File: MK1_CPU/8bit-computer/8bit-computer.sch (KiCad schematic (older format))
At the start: 16 parts, among them J1 USB_B-8bit-computer-rescue, J2 Barrel_Jack_Switch, U1 74HCT32, U2 74HCT32

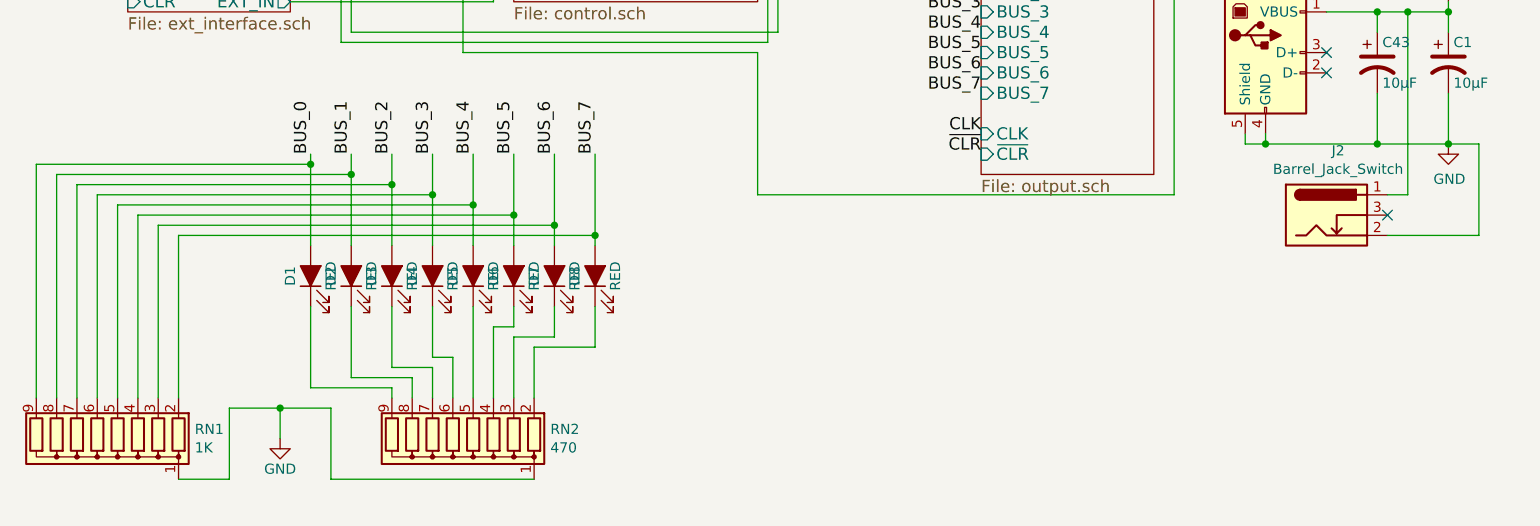
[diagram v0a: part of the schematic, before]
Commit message: 2.0b hardware revision
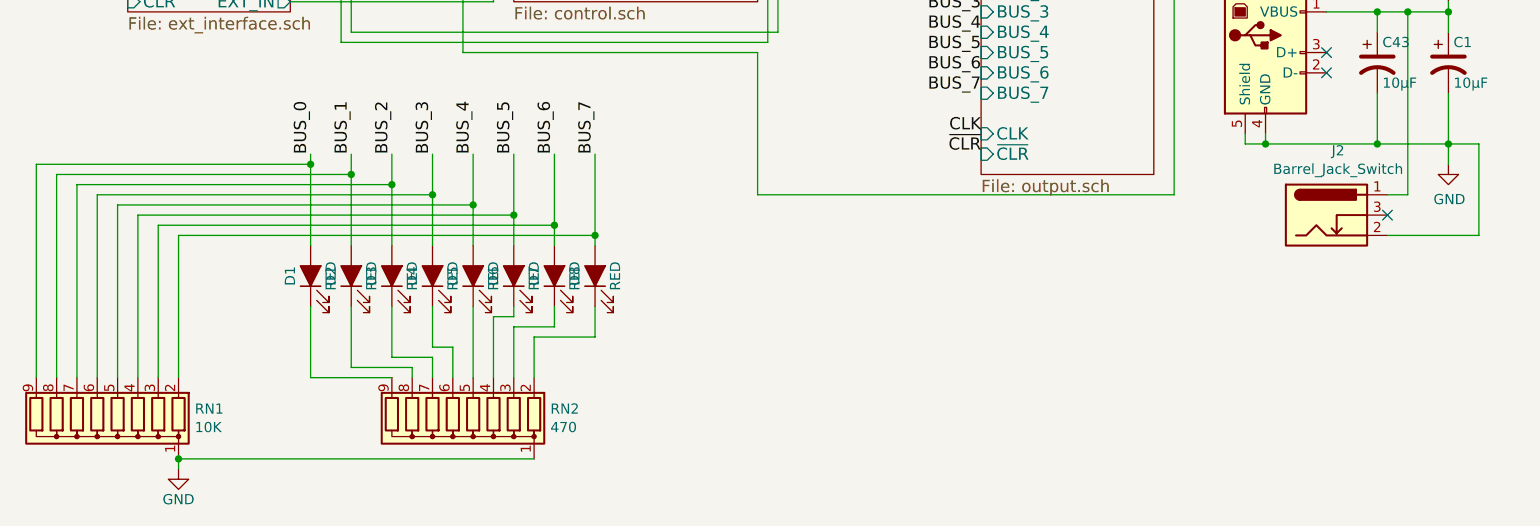
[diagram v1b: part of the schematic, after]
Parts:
- RN1: value 1K -> 10K
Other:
- moved on the sheet: RN1, RN2
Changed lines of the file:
@@
 L power:GND #PWR01
 U 1 1 5B60DD27
-P 1800 10850
-F 0 "#PWR01" H 1800 10600 50  0001 C CNN
-F 1 "GND" H 1800 10700 50  0000 C CNN
-F 2 "" H 1800 10850 50  0001 C CNN
-F 3 "" H 1800 10850 50  0001 C CNN
-	1    1800 10850
+P 1300 11000
+F 0 "#PWR01" H 1300 10750 50  0001 C CNN
+F 1 "GND" H 1300 10850 50  0000 C CNN
+F 2 "" H 1300 11000 50  0001 C CNN
+F 3 "" H 1300 11000 50  0001 C CNN
+	1    1300 11000
 	1    0    0    -1
 $EndComp
-Wire Wire Line
-	1800 10850 1800 10700
 Wire Wire Line
 	2350 9600 2350 9900
@@
 L power:GND #PWR03
 U 1 1 5E907257
-P 7550 9400
-F 0 "#PWR03" H 7550 9150 50  0001 C CNN
-F 1 "GND" H 7555 9227 50  0000 C CNN
-F 2 "" H 7550 9400 50  0001 C CNN
-F 3 "" H 7550 9400 50  0001 C CNN
-	1    7550 9400
+P 7550 9500
+F 0 "#PWR03" H 7550 9250 50  0001 C CNN
+F 1 "GND" H 7555 9327 50  0000 C CNN
+F 2 "" H 7550 9500 50  0001 C CNN
+F 3 "" H 7550 9500 50  0001 C CNN
+	1    7550 9500
 	1    0    0    -1
 $EndComp
@@
 Wire Wire Line
 	650  5200 950  5200
-$Comp
-L Device:R_Network08 RN2
-U 1 1 76216E60
-P 2650 10850
-F 0 "RN2" H 2170 10804 50  0000 R CNN
-F 1 "470" H 2170 10895 50  0000 R CNN
-F 2 "Resistor_THT:R_Array_SIP9" V 3125 10850 50  0001 C CNN
-F 3 "http://www.vishay.com/docs/31509/csc.pdf" H 2650 10850 50  0001 C CNN
-	1    2650 10850
-	-1   0    0    1
-$EndComp
-Wire Wire Line
-	3050 11050 2050 11050
-Wire Wire Line
-	2050 11050 2050 10700
-Wire Wire Line
-	2050 10700 1800 10700
-Wire Wire Line
-	1950 10600 2350 10600
-Wire Wire Line
-	2350 10600 2350 10650
-Wire Wire Line
-	1950 10200 1950 10600
-Wire Wire Line
-	2150 10550 2450 10550
-Wire Wire Line
-	2450 10550 2450 10650
-Wire Wire Line
-	2150 10200 2150 10550
-Wire Wire Line
-	2350 10500 2550 10500
-Wire Wire Line
-	2550 10500 2550 10650
-Wire Wire Line
-	2350 10200 2350 10500
-Wire Wire Line
-	2550 10450 2650 10450
-Wire Wire Line
-	2650 10450 2650 10650
-Wire Wire Line
-	2550 10200 2550 10450
-Wire Wire Line
-	2750 10200 2750 10650
-Wire Wire Line
-	2950 10300 2950 10200
-Wire Wire Line
-	2950 10300 2850 10300
-Wire Wire Line
-	2850 10300 2850 10650
-Wire Wire Line
-	3150 10350 2950 10350
-Wire Wire Line
-	2950 10350 2950 10650
-Wire Wire Line
-	3150 10200 3150 10350
-Wire Wire Line
-	3350 10400 3050 10400
-Wire Wire Line
-	3050 10400 3050 10650
-Wire Wire Line
-	3350 10200 3350 10400
+Wire Wire Line
+	1950 10550 2350 10550
+Wire Wire Line
+	1950 10200 1950 10550
+Wire Wire Line
+	2150 10500 2450 10500
+Wire Wire Line
+	2450 10500 2450 10550
+Wire Wire Line
+	2150 10200 2150 10500
+Wire Wire Line
+	2350 10450 2550 10450
+Wire Wire Line
+	2550 10450 2550 10550
+Wire Wire Line
+	2350 10200 2350 10450
+Wire Wire Line
+	2550 10400 2650 10400
+Wire Wire Line
+	2650 10400 2650 10550
+Wire Wire Line
+	2550 10200 2550 10400
+Wire Wire Line
+	2750 10200 2750 10550
+Wire Wire Line
+	2950 10250 2950 10200
+Wire Wire Line
+	2950 10250 2850 10250
+Wire Wire Line
+	2850 10250 2850 10550
+Wire Wire Line
+	3150 10300 2950 10300
+Wire Wire Line
+	2950 10300 2950 10550
+Wire Wire Line
+	3150 10200 3150 10300
+Wire Wire Line
+	3350 10350 3050 10350
+Wire Wire Line
+	3050 10350 3050 10550
+Wire Wire Line
+	3350 10200 3350 10350
 Wire Wire Line
 	7450 7950 7750 7950
@@
 Wire Wire Line
 	2200 8050 2950 8050
-$Comp
-L Device:R_Network08 RN1
-U 1 1 7674F9C0
-P 900 10850
-F 0 "RN1" H 420 10804 50  0000 R CNN
-F 1 "1K" H 420 10895 50  0000 R CNN
-F 2 "Resistor_THT:R_Array_SIP9" V 1375 10850 50  0001 C CNN
-F 3 "http://www.vishay.com/docs/31509/csc.pdf" H 900 10850 50  0001 C CNN
-	1    900  10850
-	-1   0    0    1
-$EndComp
-Wire Wire Line
-	1300 11050 1550 11050
-Wire Wire Line
-	1550 11050 1550 10700
-Wire Wire Line
-	1550 10700 1800 10700
-Connection ~ 1800 10700
-Wire Wire Line
-	600  9500 600  10650
-Wire Wire Line
-	700  9550 700  10650
-Wire Wire Line
-	800  9600 800  10650
-Wire Wire Line
-	900  9650 900  10650
-Wire Wire Line
-	1000 9700 1000 10650
-Wire Wire Line
-	1100 9750 1100 10650
-Wire Wire Line
-	1200 9800 1200 10650
-Wire Wire Line
-	1300 9850 1300 10650
 Text Notes 3750 2300 2    60   ~ 0
 STK
@@
 Text Label 6450 6550 2    60   ~ 0
 ~CLR
+Wire Wire Line
+	600  9500 600  10550
+Wire Wire Line
+	700  9550 700  10550
+Wire Wire Line
+	800  9600 800  10550
+Wire Wire Line
+	900  9650 900  10550
+Wire Wire Line
+	1000 9700 1000 10550
+Wire Wire Line
+	1100 9750 1100 10550
+Wire Wire Line
+	1200 9800 1200 10550
+Wire Wire Line
+	1300 9850 1300 10550
+$Comp
+L Device:R_Network08 RN1
+U 1 1 7674F9C0
+P 900 10750
+F 0 "RN1" H 420 10704 50  0000 R CNN
+F 1 "10K" H 420 10795 50  0000 R CNN
+F 2 "Resistor_THT:R_Array_SIP9" V 1375 10750 50  0001 C CNN
+F 3 "http://www.vishay.com/docs/31509/csc.pdf" H 900 10750 50  0001 C CNN
+	1    900  10750
+	-1   0    0    1
+$EndComp
+Wire Wire Line
+	1300 11000 1300 10950
+$Comp
+L Device:R_Network08 RN2
+U 1 1 76216E60
+P 2650 10750
+F 0 "RN2" H 2170 10704 50  0000 R CNN
+F 1 "470" H 2170 10795 50  0000 R CNN
+F 2 "Resistor_THT:R_Array_SIP9" V 3125 10750 50  0001 C CNN
+F 3 "http://www.vishay.com/docs/31509/csc.pdf" H 2650 10750 50  0001 C CNN
+	1    2650 10750
+	-1   0    0    1
+$EndComp
+Wire Wire Line
+	1300 10950 3050 10950
+Connection ~ 1300 10950
+Wire Wire Line
+	7550 9500 7550 9400
 $EndSCHEMATC
